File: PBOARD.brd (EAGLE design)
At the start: 80 x 46 mm, 11 parts, among them J1 POWER_JACKPTH_SLOTS, J10 POWER_JACKPTH_SLOTS, J2 POWER_JACKPTH_SLOTS, J3 POWER_JACKPTH_SLOTS, J4 POWER_JACKPTH_SLOTS, J5 POWER_JACKPTH_SLOTS, J7 POWER_JACKPTH_SLOTS, J8 POWER_JACKPTH_SLOTS, J9 POWER_JACKPTH_SLOTS

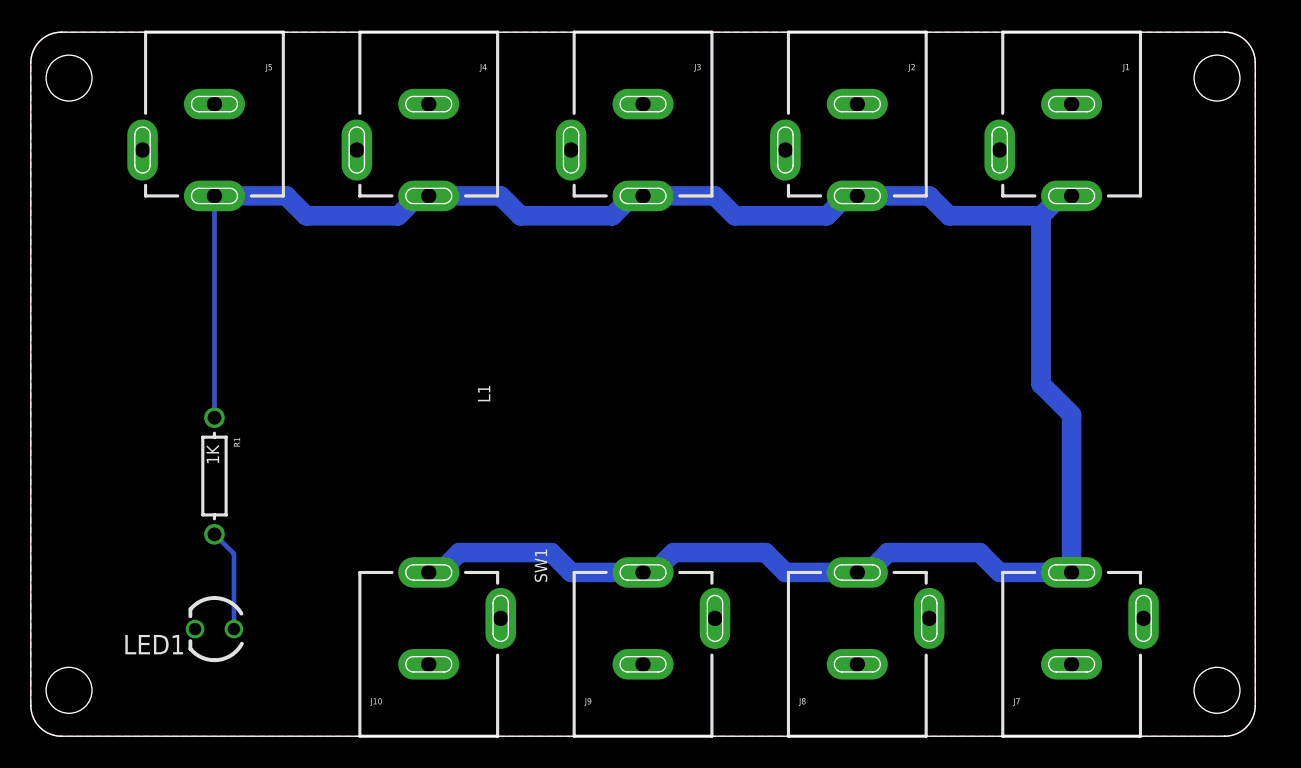
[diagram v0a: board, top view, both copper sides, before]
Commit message: Merged files from PowerDistributionBoard project
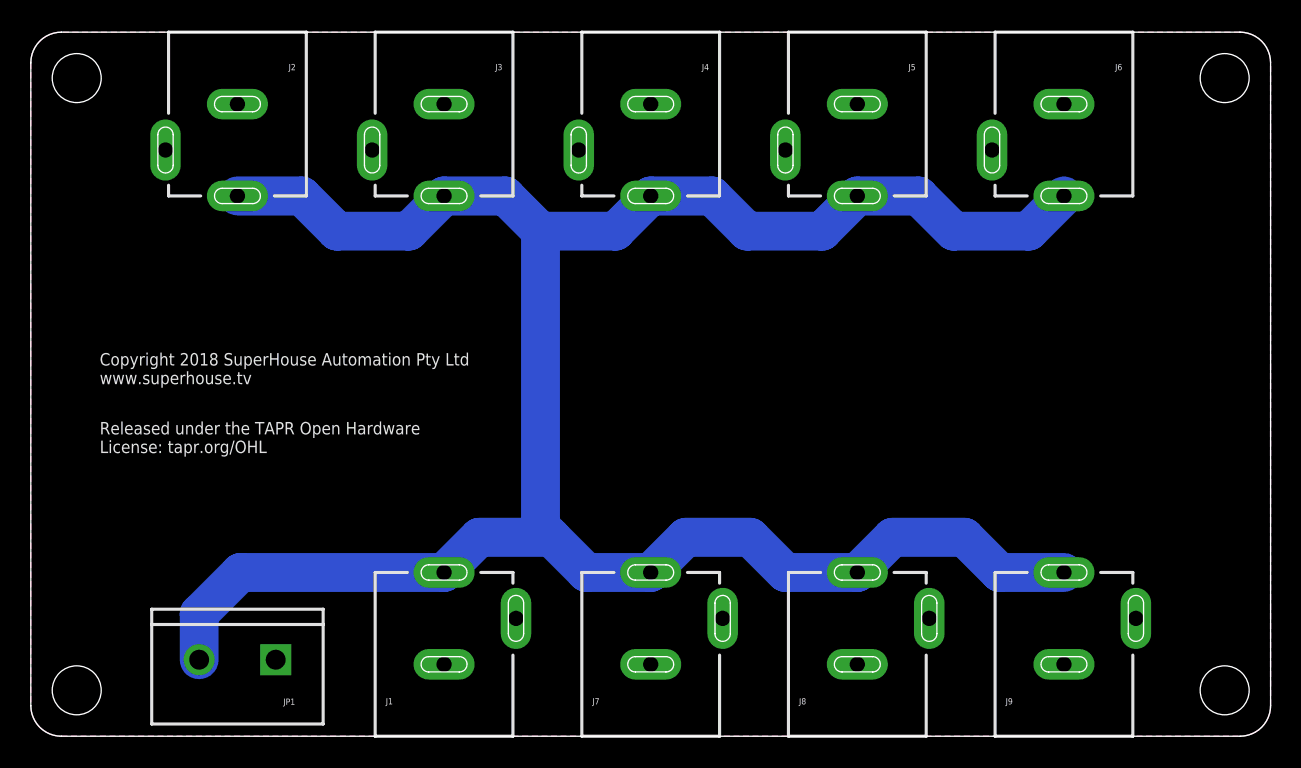
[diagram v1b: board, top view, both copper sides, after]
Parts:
- removed J10: POWER_JACKPTH_SLOTS, freetronics-jon:POWER_JACK_PTH_SLOTS
- removed LED1: GREEN, freetronics-jon:LED3MM
- removed R1: 1K, freetronics-jon:AXIAL-0.3
- added J6: POWER_JACKPTH_SLOTS, freetronics-jon:POWER_JACK_PTH_SLOTS
- added JP1: (no value), freetronics-jon:SCREWTERMINAL-5MM-2
- moved J1 66.2 mm to (27.0, -3.00), turned to 0 degrees
- moved J5 42.0 mm to (54.0, 49.0)
- moved J2 40.5 mm to (13.5, 49.0)
- moved J7 27.5 mm to (40.5, -3.00)
- moved J9 27.5 mm to (67.5, -3.00)
- moved J4 14.5 mm to (40.5, 49.0)
- moved J3 13.0 mm to (27.0, 49.0)
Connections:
- removed net 3.3V: J1.PWR, J10.PWR, J2.PWR, J3.PWR, J4.PWR, J5.PWR, J7.PWR, J8.PWR, J9.PWR, R1.P$1
- removed net N$1: LED1.A, R1.P$2
- new net VCC: J1.PWR, J2.PWR, J3.PWR, J4.PWR, J5.PWR, J6.PWR, J7.PWR, J8.PWR, J9.PWR, JP1.2
- net GND: now also J6.GND, J6.GNDBREAK, JP1.1; no longer J10.GND, J10.GNDBREAK, LED1.K
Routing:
- net VCC: track 0.00 -> 148.2 mm
- net 3.3V: track 144.2 -> 0.00 mm
- net N$1: track 6.72 -> 0.00 mm
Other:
- board size 80 x 46 mm -> 81 x 46 mm
- board text added: "Copyright 2018 SuperHouse Automation Pty Ltd www.superhouse.tv"
- board text added: "Released under the TAPR Open Hardware License: tapr.org/OHL"
- board text removed: "+"
- board text removed: "-"
- board text removed: "1"
- board text removed: "2"
- board text removed: "3"
- board text removed: "4"
- board text removed: "5V FTDI"
- board text removed: "7.4V LiPo"
- board text removed: "A0: CH1 A1: CH2 A2: CH3 A3: CH4 A6: VBAT"
- board text removed: "ATmega328P 16MHz"
- board text removed: "AntBrain"
- board text removed: "D11: LA D12: LB D9: RA D10: RB D13: LED"
- board text removed: "D13"
- board text removed: "L1"
- board text removed: "PWR"
- board text removed: "SW1"
- board text removed: "SWITCH"
- board text removed: "Select "Arduino Uno" in Arduino IDE"
- board text removed: "freetronics"
- board text removed: "tron.cc/antbrain"
